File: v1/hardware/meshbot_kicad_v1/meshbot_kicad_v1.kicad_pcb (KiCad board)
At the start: 2 copper layers, 51.9 x 23.2 mm, 9 parts, among them J1 Conn_01x02_Socket, J2 Conn_01x04_Pin, J3 Conn_01x04_Pin, J4 Conn_01x01_Socket, SW1 SW_Push, U1 wio-sx1262, U2 nice_nano_clean

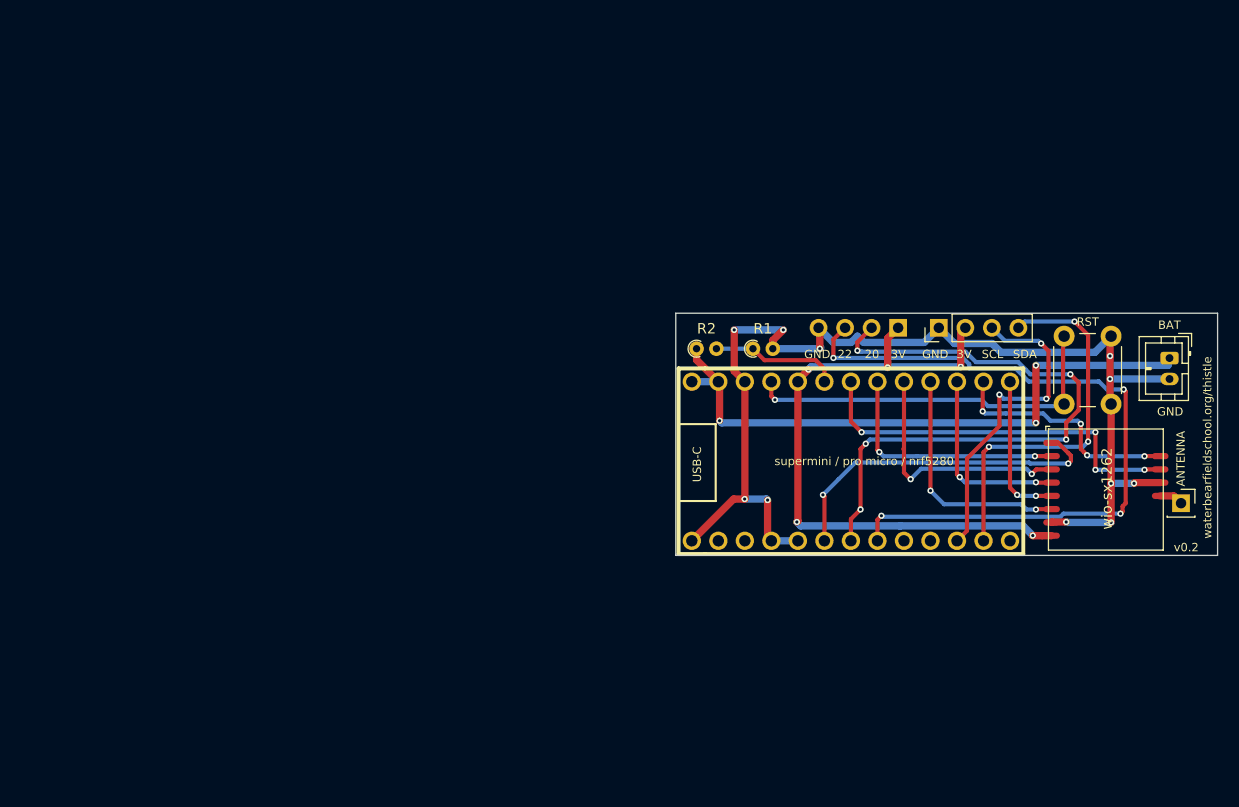
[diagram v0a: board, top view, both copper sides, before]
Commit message: update
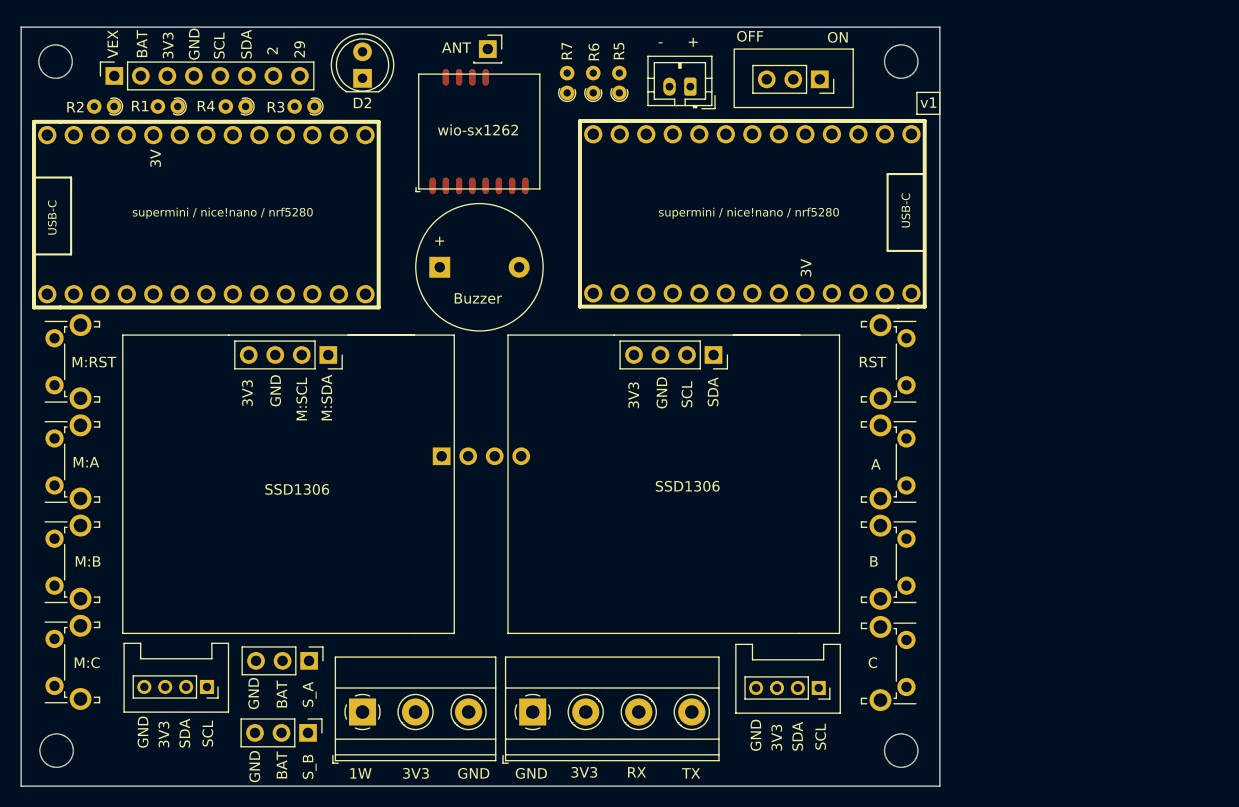
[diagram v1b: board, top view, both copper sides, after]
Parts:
- added D2: LED, LED_THT:LED_D5.0mm, F.Cu at (29.4, 1.60)
- added H1: MountingHole, MountingHole:MountingHole_3.2mm_M3, F.Cu at (0.00, 0.00)
- added H2: MountingHole, MountingHole:MountingHole_3.2mm_M3, F.Cu at (81.0, 0.00)
- added H3: MountingHole, MountingHole:MountingHole_3.2mm_M3, F.Cu at (81.0, 66.0)
- added H4: MountingHole, MountingHole:MountingHole_3.2mm_M3, F.Cu at (0.10, 66.0)
- added J11: Conn_01x03_Pin, Connector_PinHeader_2.54mm:PinHeader_1x03_P2.54mm_Vertical, F.Cu at (24.3, 57.4)
- added J12: Conn_01x03_Pin, Connector_PinHeader_2.54mm:PinHeader_1x03_P2.54mm_Vertical, F.Cu at (24.2, 64.3)
- added J13: Conn_01x08_Socket, Connector_PinSocket_2.54mm:PinSocket_1x08_P2.54mm_Vertical, F.Cu at (5.62, 1.38)
- added J5: Conn_01x04_Pin, footprints:ssd1306_a, F.Cu at (63.0, 28.1)
- added J6: Screw_Terminal_01x04, TerminalBlock_Phoenix:TerminalBlock_Phoenix_MKDS-1,5-4-5.08_1x04_P5.08mm_Horizontal, F.Cu at (45.7, 62.3)
- added J7: Screw_Terminal_01x03, TerminalBlock_Phoenix:TerminalBlock_Phoenix_MKDS-1,5-3-5.08_1x03_P5.08mm_Horizontal, F.Cu at (29.4, 62.3)
- added J8: Conn_01x03_Socket, footprints:usual_switch, F.Cu at (73.2, 1.70)
- added J9: Conn_01x02_Socket, Buzzer_Beeper:Buzzer_12x9.5RM7.6, F.Cu at (36.8, 19.7)
- added R3: R, Resistor_THT:R_Axial_DIN0204_L3.6mm_D1.6mm_P1.90mm_Vertical, F.Cu at (24.8, 4.30)
- added R4: R, Resistor_THT:R_Axial_DIN0204_L3.6mm_D1.6mm_P1.90mm_Vertical, F.Cu at (18.2, 4.30)
- added R5: R, Resistor_THT:R_Axial_DIN0204_L3.6mm_D1.6mm_P1.90mm_Vertical, F.Cu at (54.0, 3.00)
- added R6: R, Resistor_THT:R_Axial_DIN0204_L3.6mm_D1.6mm_P1.90mm_Vertical, F.Cu at (51.5, 3.00)
- added R7: R, Resistor_THT:R_Axial_DIN0204_L3.6mm_D1.6mm_P1.90mm_Vertical, F.Cu at (49.0, 3.00)
- added SW2: SW_Push, Button_Switch_THT:SW_Tactile_SPST_Angled_PTS645Vx31-2LFS, F.Cu at (-0.10, 40.6)
- added SW3: SW_Push, Button_Switch_THT:SW_Tactile_SPST_Angled_PTS645Vx31-2LFS, F.Cu at (81.5, 26.5)
- added SW4: SW_Push, Button_Switch_THT:SW_Tactile_SPST_Angled_PTS645Vx31-2LFS, F.Cu at (81.5, 36.1)
- added SW5: SW_Push, Button_Switch_THT:SW_Tactile_SPST_Angled_PTS645Vx31-2LFS, F.Cu at (81.5, 45.7)
- added SW6: SW_Push, Button_Switch_THT:SW_Tactile_SPST_Angled_PTS645Vx31-2LFS, F.Cu at (81.5, 55.4)
- added SW7: SW_Push, Button_Switch_THT:SW_Tactile_SPST_Angled_PTS645Vx31-2LFS, F.Cu at (-0.10, 50.2)
- added SW8: SW_Push, Button_Switch_THT:SW_Tactile_SPST_Angled_PTS645Vx31-2LFS, F.Cu at (-0.10, 59.8)
- added U3: nice_nano_clean, footprints:nice_nano_cleanest, F.Cu at (65.5, 14.6)
- added U4: grove_a, footprints:grove_a, F.Cu at (14.5, 59.9)
- added U5: grove_a, footprints:grove_rightangle, F.Cu at (73.1, 60.0)
- J2: footprint Connector_PinHeader_2.54mm:PinHeader_1x04_P2.54mm_Vertical -> footprints:gps_ublox_blue
- J3: footprint Connector_PinHeader_2.54mm:PinHeader_1x04_P2.54mm_Vertical -> footprints:ssd1306_a
- SW1: footprint Button_Switch_THT:SW_PUSH_6mm -> Button_Switch_THT:SW_Tactile_SPST_Angled_PTS645Vx31-2LFS
- moved SW1 96.7 mm to (-0.10, 31.0)
- moved J4 79.4 mm to (41.4, -1.20)
- moved U2 66.1 mm to (15.7, 14.7)
- moved U1 64.6 mm to (34.8, 12.2), turned to 0 degrees
- moved R2 60.4 mm to (5.60, 4.30), turned to 180 degrees
- moved R1 59.8 mm to (11.7, 4.30), turned to 180 degrees
- moved J3 58.5 mm to (26.1, 28.1), turned to -90 degrees
- moved J1 52.8 mm to (60.8, 2.40), turned to 180 degrees
- moved J2 45.4 mm to (37.0, 37.8), turned to -90 degrees
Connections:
- net BATT_MEASURE renamed MESH_BATT_MEASURE
- net MICRO_RST renamed MESH_RST
- net SCL renamed SCL_MESH
- net SDA renamed SDA_MESH
- J1 pad 1: BAT -> V_EXT
- J3 pad 1: GND -> 3V3
- J3 pad 2: 3V3 -> GND
- U2 pad 1: unconnected-(U2-TX0/P0.06-Pad1) -> MESH_TX
- U2 pad 12: unconnected-(U2-P1.06-Pad12) -> MESH_BUTTON_C
- U2 pad 2: unconnected-(U2-RX1/P0.08-Pad2) -> MESH_RX
- U2 pad 8: unconnected-(U2-P0.24-Pad8) -> MESH_BUTTON_A
- U2 pad 9: unconnected-(U2-P1.00-Pad9) -> MESH_BUTTON_B
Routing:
- net GND: track 111.4 -> 0.00 mm, vias 11 -> 0
- net GPS_TX: track 70.5 -> 0.00 mm, vias 4 -> 0
- net 3V3: track 62.9 -> 0.00 mm, vias 5 -> 0
- net GPS_RX: track 60.5 -> 0.00 mm, vias 5 -> 0
- net BAT: track 59.6 -> 0.00 mm, vias 3 -> 0
- net BUSY: track 37.5 -> 0.00 mm, vias 4 -> 0
- net SDA_MESH: track 36.6 -> 0.00 mm, vias 3 -> 0
- net MESH_RST: track 36.5 -> 0.00 mm, vias 1 -> 0
- net RF_SW: track 32.5 -> 0.00 mm, vias 2 -> 0
- net SCL_MESH: track 31.4 -> 0.00 mm, vias 3 -> 0
- net MOSI: track 24.0 -> 0.00 mm, vias 2 -> 0
- net MISO: track 23.5 -> 0.00 mm, vias 2 -> 0
- net DIO1: track 23.1 -> 0.00 mm, vias 4 -> 0
- net CS: track 22.8 -> 0.00 mm, vias 2 -> 0
- net SCK: track 18.3 -> 0.00 mm, vias 2 -> 0
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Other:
- board size 51.9 x 23.2 mm -> 88 x 72.7 mm
- board text added: "+"
- board text added: "-"
- board text added: "1W"
- board text added: "2"
- board text added: "29"
- board text added: "3V3"
- board text added: "A"
- board text added: "ANT"
- board text added: "B"
- board text added: "Buzzer"
- board text added: "C"
- board text added: "GPS_RX"
- board text added: "GPS_TX"
- board text added: "M:A"
- board text added: "M:B"
- board text added: "M:C"
- board text added: "M:RST"
- board text added: "M:SCL"
- board text added: "M:SDA"
- board text added: "MESHBOT VER 1"
- board text added: "OFF"
- board text added: "ON"
- board text added: "RX"
- board text added: "SSD1306"
- board text added: "S_A"
- board text added: "S_B"
- board text added: "TX"
- board text added: "VEX"
- board text added: "edgecollective.io/meshbot"
- board text added: "v1"
- board text removed: "20"
- board text removed: "22"
- board text removed: "ANTENNA"
- board text removed: "v0.2"
- board text removed: "waterbearfieldschool.org/thistle"
